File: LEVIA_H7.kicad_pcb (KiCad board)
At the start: 6 copper layers, 36.7 x 36.7 mm, 135 parts, among them J1 TF-028-H265, Q1 AO3400A, SW1 SW_Push, U1 USBLC6-2P6, U10 ZX-SH1.0-4PWT, U11 ZX-SH1.0-3PWT, U12 SIT1051TK/3, U13 ZX-SH1.0-4PWT, U14 ICM-42688-P, U15 ICM-42688-P, U16 DPS368XTSA1, U17 IST8310, U18 ZX-SH1.0-4PWT, U19 ZX-SH1.0-6PWT, U2 STM32H743VIHx, U20 ZX-SH1.0-6PWT, U21 ZX-SH1.0-3PWT, U22 ZX-SH1.0-8PWT, U3 ZX-SH1.0-4PWT, U4 LMR43620R5RPER, U5 LMR604303SRAKRQ1, U6 AP7361C-33FGE-7, U7 AP7361C-33FGE-7, U8 ZX-SH1.0-4PWT, U9 AT7456ELAH, Y1 8MHz, Y2 XL7EL89COI-111YLC-27M

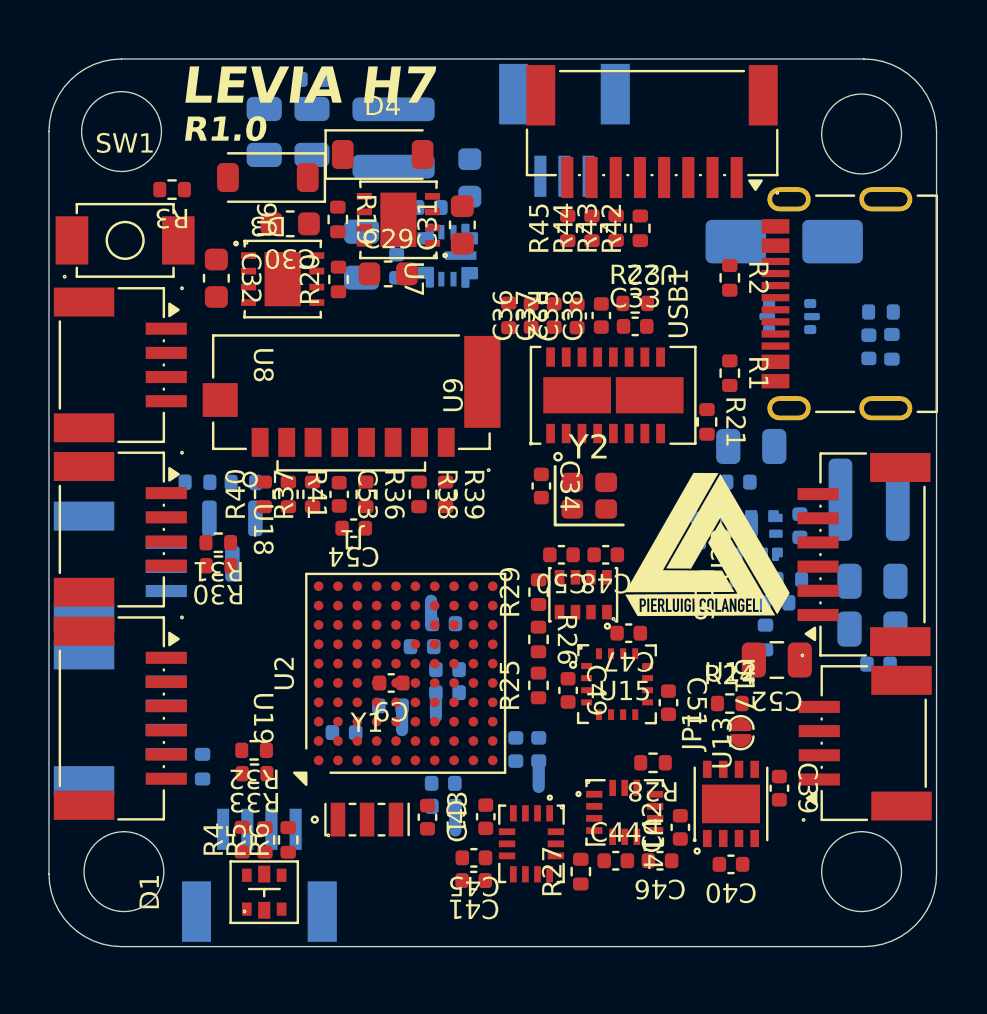
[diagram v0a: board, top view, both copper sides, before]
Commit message: MORE LAYOUT TESTS
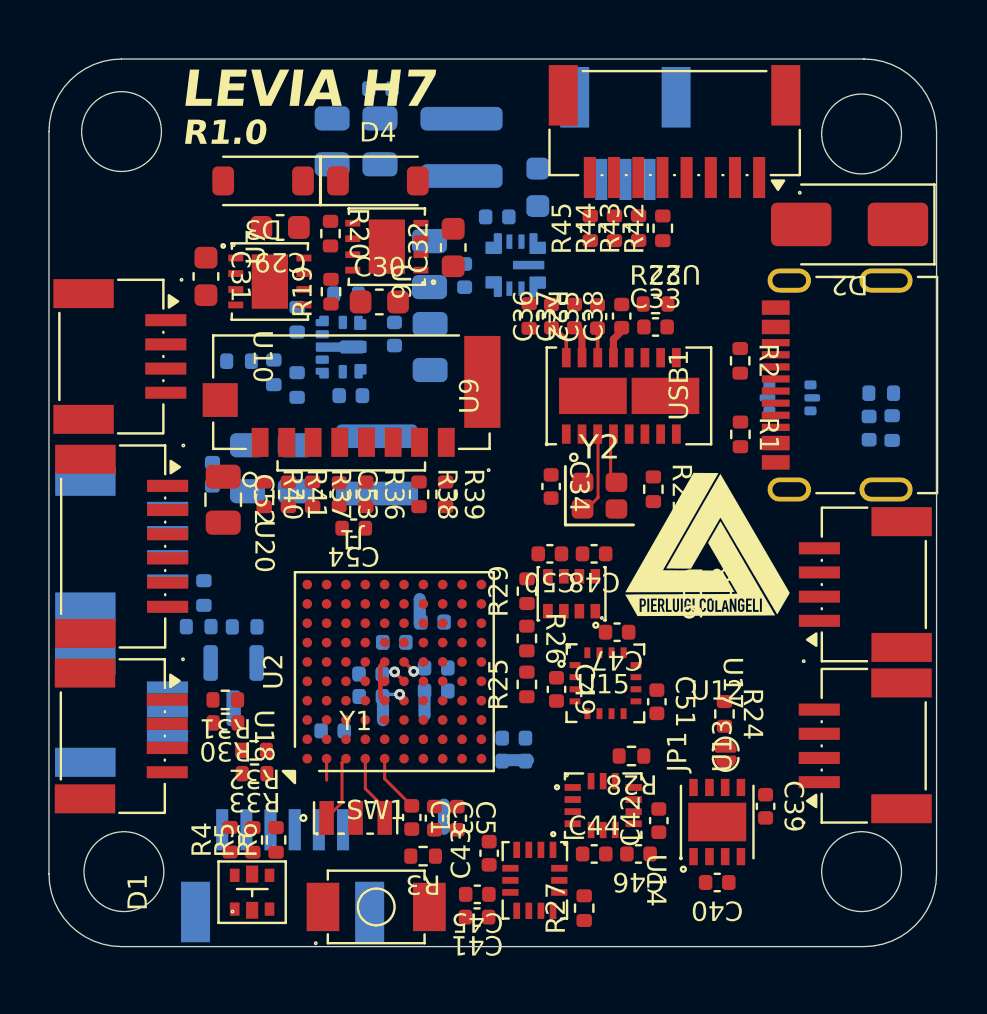
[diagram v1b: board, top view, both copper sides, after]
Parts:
- removed REF**: OSHW-Logo2_9.8x8mm_SilkScreen, Symbol:OSHW-Logo2_9.8x8mm_SilkScreen
- removed REF**: KiCad-Logo2_5mm_SilkScreen, Symbol:KiCad-Logo2_5mm_SilkScreen
- C3, C5, D2, U10: moved to F.Cu
- C9, U19: moved to B.Cu
- moved U8 31.7 mm to (154.0, 72.6), turned to 90 degrees
- moved U20 30.3 mm to (123.7, 71.0), turned to -90 degrees
- moved R3 29.4 mm to (135.9, 83.8)
- moved SW1 29.4 mm to (134.0, 85.9)
- moved C28 28.6 mm to (127.2, 68.0), turned to 90 degrees
- moved C25 26.7 mm to (128.7, 67.8), turned to 90 degrees
- moved R16 24.6 mm to (128.3, 63.3), turned to 180 degrees
- moved C27 24.3 mm to (130.7, 67.8), turned to 90 degrees
- moved C52 23.8 mm to (127.7, 69.1), turned to -90 degrees
- moved R15 22.9 mm to (129.8, 63.8), turned to -90 degrees
- moved U10 22.0 mm to (123.6, 63.1), turned to -90 degrees
- moved R9 21.9 mm to (130.7, 64.3), turned to -90 degrees
- moved R12 20.7 mm to (130.7, 61.6), turned to 90 degrees
- moved L2 20.4 mm to (134.0, 67.6), turned to -90 degrees
- moved C21 19.3 mm to (132.9, 64.8), turned to 0 degrees
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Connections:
- net /DIGITAL VTX/UART2.TX renamed /MCU/UART2.TX
- U1 pad 4: /MCU/USB_OTG_P.DM -> /USB_OTG_P.DM
- U2 pad A4: /MCU/UART4.TX -> /DIGITAL VTX/UART4.TX
- U2 pad B4: /MCU/UART4.RX -> /DIGITAL VTX/UART4.RX
- U2 pad C10: /MCU/USB_OTG_P.DM -> /MCU/USB_OTG_P.DN
- U2 pad C6: /DIGITAL VTX/UART2.RX -> /MCU/UART2.RX
- U20 pad 3: /DIGITAL VTX/UART3.TX -> /DIGITAL VTX/UART4.TX
- U20 pad 4: /DIGITAL VTX/UART3.RX -> /DIGITAL VTX/UART4.RX
- U20 pad 6: /DIGITAL VTX/UART2.RX -> /DIGITAL VTX/UART3.RX
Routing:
- net Net-(U9-CLKIN): track 0.00 -> 3.46 mm
- net /MCU/OSC_OUT: track 0.00 -> 2.78 mm
- net /MCU/OSC_IN: track 0.00 -> 2.78 mm
- net /MCU/NRST: track 0.00 -> 2.41 mm
- net Net-(U9-XFB): track 0.00 -> 2.14 mm
- net GND: track 0.00 -> 1.75 mm
- net Net-(U9-VOUT): track 0.00 -> 1.45 mm
- net Net-(U9-VIN): track 0.00 -> 1.44 mm
- net Net-(U9-SAG): track 0.00 -> 1.30 mm
- net +5V_SYS: track 0.00 -> 1.30 mm
- net /MCU/VDD: track 0.00 -> 1.10 mm, vias 0 -> 1
- net /MCU/VDD_LDO: track 0.00 -> 1.08 mm, vias 0 -> 1
- net /MCU/VDD_USB: track 0.00 -> 1.07 mm, vias 0 -> 1
- net /MCU/SPI1.CS: track 0.00 -> 0.89 mm
